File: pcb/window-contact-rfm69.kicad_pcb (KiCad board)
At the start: 2 copper layers, 35.4 x 36.6 mm, 25 parts, among them IC1 ATMEGA328P-A, P1 VCC, P2 TX/RX, P3 RE1, P4 ISP, P5 RE2, P6 AN, P7 RE3, SW1 LED ON

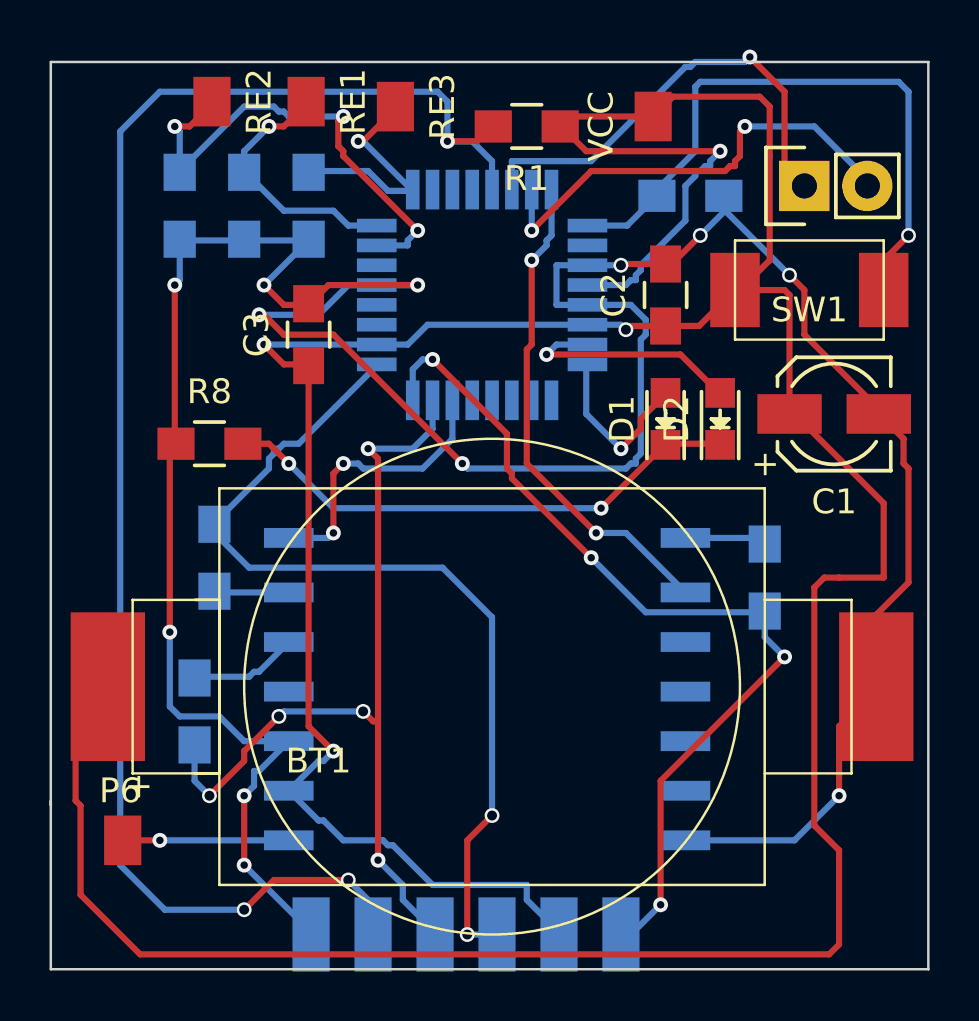
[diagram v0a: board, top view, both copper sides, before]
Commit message: finial version for allpcb
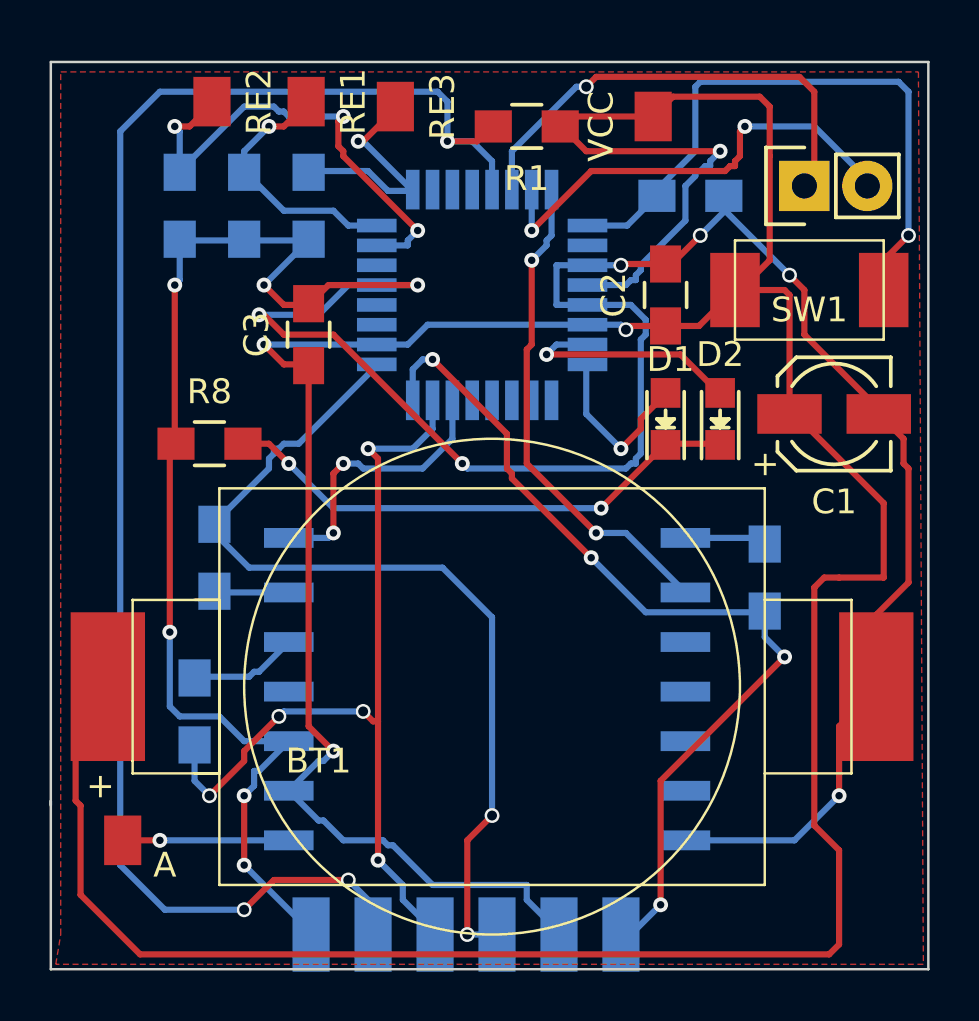
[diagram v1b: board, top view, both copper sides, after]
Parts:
- renumbered P6 to A
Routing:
- net Net-(IC1-Pad30): track 18.6 -> 20.3 mm
- added copper zone on F.Cu, net GND
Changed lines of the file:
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@@
     (links 53)
     (no_connects 0)
-    (area 162.2 122.6 197.8 160)
+    (area 162.349999 123.149999 197.850001 159.850001)
     (thickness 1.6)
     (drawings 5)
-    (tracks 400)
+    (tracks 399)
     (zones 0)
     (modules 25)
@@
     (last_trace_width 0.25)
     (trace_clearance 0.2)
-    (zone_clearance 0.508)
+    (zone_clearance 0.708)
     (zone_45_only no)
     (trace_min 0.2)
@@
     (fp_line (start -6 7) (end -6 -9) (layer F.SilkS) (width 0.1))
     (fp_line (start -6 -9) (end 16 -9) (layer F.SilkS) (width 0.1))
-    (fp_text user + (at -9.25 3) (layer F.SilkS)
+    (fp_text user + (at -10.8 3) (layer F.SilkS)
       (effects (font (size 1 1) (thickness 0.15)))
     )
@@
     (tags "LED 0805 SMD")
     (attr smd)
-    (fp_text reference D1 (at 0 -1.75 90) (layer F.SilkS)
+    (fp_text reference D1 (at 2.4 0.2 180) (layer F.SilkS)
       (effects (font (size 1 1) (thickness 0.15)))
     )
@@
     (tags "LED 0805 SMD")
     (attr smd)
-    (fp_text reference D2 (at 0 -1.75 90) (layer F.SilkS)
+    (fp_text reference D2 (at 2.6 0 180) (layer F.SilkS)
       (effects (font (size 1 1) (thickness 0.15)))
     )
@@
   (module wirepad:Wire_SMD_Pad_1PIN (layer F.Cu)
     (at 164.2 153)
-    (fp_text reference P6 (at 1 -0.4) (layer F.SilkS)
+    (fp_text reference A (at 2.8 2.6) (layer F.SilkS)
       (effects (font (size 1 1) (thickness 0.15)))
     )
@@
     (tags "resistor 0805")
     (attr smd)
-    (fp_text reference R2 (at 0 2.1 270) (layer B.SilkS)
+    (fp_text reference R2 (at 3.4 0.4 270) (layer B.SilkS)
       (effects (font (size 1 1) (thickness 0.15)) (justify mirror))
     )
@@
     (tags "resistor 0805")
     (attr smd)
-    (fp_text reference R3 (at 0 2.1 270) (layer B.SilkS)
+    (fp_text reference R3 (at 1.6 1.6 270) (layer B.SilkS)
       (effects (font (size 1 1) (thickness 0.15)) (justify mirror))
     )
@@
     (tags "resistor 0805")
     (attr smd)
-    (fp_text reference R7 (at 0 2.1 270) (layer B.SilkS)
+    (fp_text reference R7 (at -1.8 -1.8 270) (layer B.SilkS)
       (effects (font (size 1 1) (thickness 0.15)) (justify mirror))
     )
@@
   (segment (start 173.8 142.2) (end 173.6 142.4) (width 0.25) (layer B.Cu) (net 13) (status 80000))
   (segment (start 173.6 142.4) (end 172 142.4) (width 0.25) (layer B.Cu) (net 13) (status 80000))
-  (segment (start 168.2 150.75) (end 168.2 152.2) (width 0.25) (layer B.Cu) (net 14) (status 400000))
+  (segment (start 168.2 150.75) (end 168.2 152.2) (width 0.25) (layer B.Cu) (net 14))
   (segment (start 175.4 149.8) (end 175.6 149.8) (width 0.25) (layer F.Cu) (net 14))
   (segment (start 175 149.4) (end 175.4 149.8) (width 0.25) (layer F.Cu) (net 14))
@@
   (segment (start 187 157.2) (end 185.8 158.4) (width 0.25) (layer B.Cu) (net 15) (status 80000))
   (segment (start 185.8 158.4) (end 185.4 158.4) (width 0.25) (layer B.Cu) (net 15) (status 80000))
-  (segment (start 169 141.85) (end 169 142.2) (width 0.25) (layer B.Cu) (net 16) (status C00000))
-  (segment (start 169 142.2) (end 170.4 143.6) (width 0.25) (layer B.Cu) (net 16) (status 400000))
-  (segment (start 179.2 158.4) (end 180.4 158.4) (width 0.25) (layer B.Cu) (net 16) (status 800000))
+  (segment (start 169 141.85) (end 169 142.2) (width 0.25) (layer B.Cu) (net 16))
+  (segment (start 169 142.2) (end 170.4 143.6) (width 0.25) (layer B.Cu) (net 16))
+  (segment (start 179.2 158.4) (end 180.4 158.4) (width 0.25) (layer B.Cu) (net 16))
   (via (at 179.2 158.4) (size 0.6) (drill 0.4) (layers F.Cu B.Cu) (net 16))
   (segment (start 179.2 154.6) (end 179.2 158.4) (width 0.25) (layer F.Cu) (net 16))
@@
   (segment (start 179.6 126.4) (end 180.2 125.8) (width 0.25) (layer F.Cu) (net 26) (status 80000))
   (segment (start 180.2 125.8) (end 180.25 125.8) (width 0.25) (layer F.Cu) (net 26) (status 80000))
+  (segment (start 181 128.35) (end 181 126.8) (width 0.25) (layer B.Cu) (net 27))
+  (segment (start 193.2 124.4) (end 193.2 127.8) (width 0.25) (layer F.Cu) (net 27))
+  (segment (start 192.6 123.8) (end 193.2 124.4) (width 0.25) (layer F.Cu) (net 27))
+  (segment (start 184.4 123.8) (end 192.6 123.8) (width 0.25) (layer F.Cu) (net 27))
+  (segment (start 184 124.2) (end 184.4 123.8) (width 0.25) (layer F.Cu) (net 27))
+  (via (at 184 124.2) (size 0.6) (drill 0.4) (layers F.Cu B.Cu) (net 27))
+  (segment (start 183.6 124.2) (end 184 124.2) (width 0.25) (layer B.Cu) (net 27))
+  (segment (start 181 126.8) (end 183.6 124.2) (width 0.25) (layer B.Cu) (net 27))
+  (segment (start 193.2 127.8) (end 192.8 128.2) (width 0.25) (layer F.Cu) (net 27))
   (segment (start 192.8 128.2) (end 192 127.4) (width 0.25) (layer F.Cu) (net 27) (status 80000))
-  (segment (start 192 127.4) (end 192 124.4) (width 0.25) (layer F.Cu) (net 27) (status 80000))
-  (segment (start 192 124.4) (end 190.6 123) (width 0.25) (layer F.Cu) (net 27) (status 80000))
-  (via (at 190.6 123) (size 0.6) (layers F.Cu B.Cu) (net 27) (status 80000))
-  (segment (start 190.6 123) (end 190.4 123.2) (width 0.25) (layer B.Cu) (net 27) (status 80000))
-  (segment (start 190.4 123.2) (end 188.4 123.2) (width 0.25) (layer B.Cu) (net 27) (status 80000))
-  (segment (start 188.4 123.2) (end 188.2 123.4) (width 0.25) (layer B.Cu) (net 27) (status 80000))
-  (segment (start 188.2 123.4) (end 188 123.4) (width 0.25) (layer B.Cu) (net 27) (status 80000))
-  (segment (start 188 123.4) (end 184.2 127.2) (width 0.25) (layer B.Cu) (net 27) (status 80000))
-  (segment (start 184.2 127.2) (end 181 127.2) (width 0.25) (layer B.Cu) (net 27) (status 80000))
-  (segment (start 181 127.2) (end 181 128.35) (width 0.25) (layer B.Cu) (net 27) (status 80000))
   (segment (start 195.34 128.2) (end 195.4 128.2) (width 0.25) (layer B.Cu) (net 28) (status 80000))
   (segment (start 195.4 128.2) (end 195.4 128) (width 0.25) (layer B.Cu) (net 28) (status 80000))
@@
   (segment (start 170.4 148) (end 168.2 148) (width 0.25) (layer B.Cu) (net 33) (status 80000))
   (segment (start 168.2 148) (end 168.2 148.05) (width 0.25) (layer B.Cu) (net 33) (status 80000))
+  (zone (net 2) (net_name GND) (layer F.Cu) (hatch edge 0.508)
+    (connect_pads (clearance 0.708))
+    (min_thickness 0.254)
+    (fill yes (arc_segments 16) (thermal_gap 0.508) (thermal_bridge_width 0.508))
+    (polygon
+      (pts
+        (xy 162.8 123.6) (xy 197.4 123.6) (xy 197.6 159.6) (xy 162.6 159.6) (xy 162.8 158.4)
+      )
+    )
+  )
 )
